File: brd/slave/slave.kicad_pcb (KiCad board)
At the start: 2 copper layers, 43.2 x 25.4 mm, 23 parts, among them P1 CONN_3X2, P2 CONN_8, P3 CONN_2, P4 CONN_6, P5 CONN_1, Q1 BC847, U1 LM78L05ACZ, U2 ATMEGA328P-A, X1 16MHz

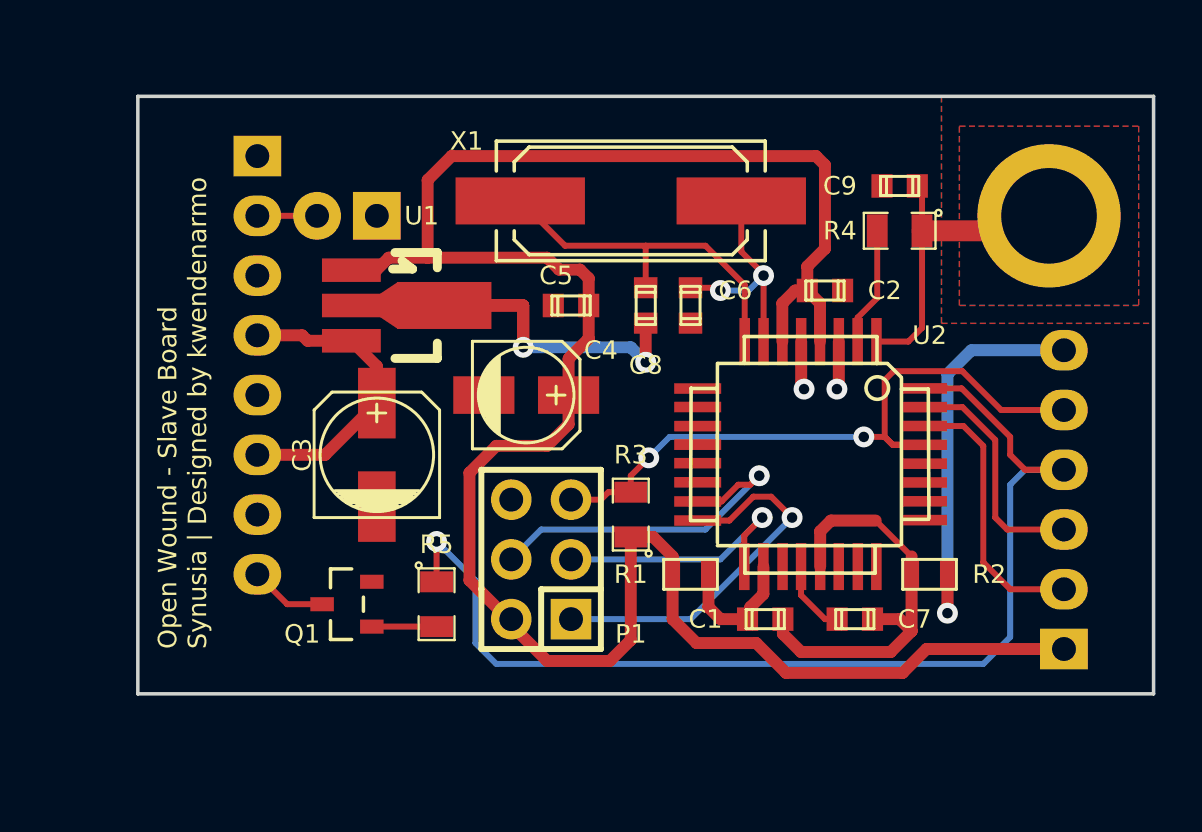
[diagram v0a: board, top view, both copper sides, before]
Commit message: slave version rc3
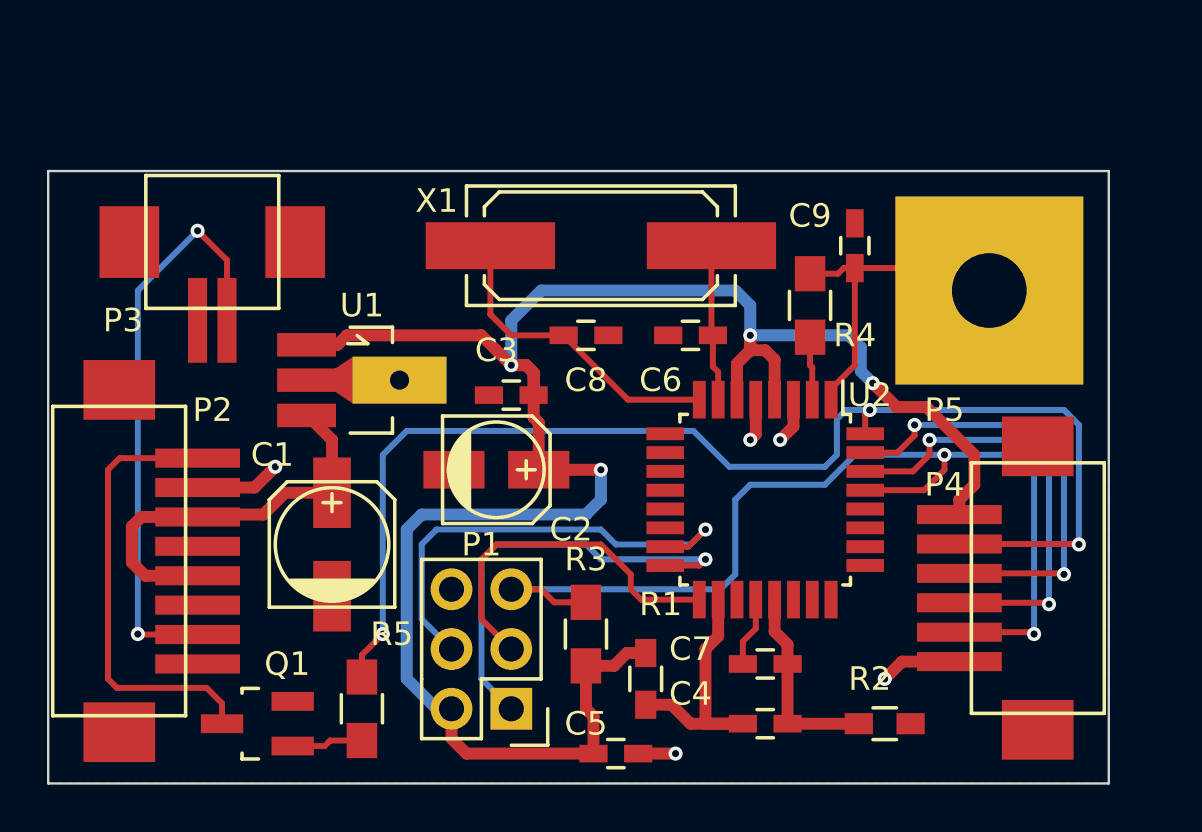
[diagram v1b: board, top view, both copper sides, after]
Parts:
- added REF**: Symbol_OSHW-Logo_SilkScreen, Symbols:Symbol_OSHW-Logo_SilkScreen, B.Cu at (157.5, 103.5)
- C1: value 100nF -> 10uF; footprint Capacitors_SMD:c_0603 -> Capacitors_SMD:c_elec_5x5.3
- C2: value 100nF -> 1uF; footprint Capacitors_SMD:c_0603 -> Capacitors_SMD:c_elec_4x5.3
- C3: value 10uF -> 10nF; footprint Capacitors_SMD:c_elec_5x5.3 -> Capacitors_SMD:C_0603_HandSoldering
- C4: value 1uF -> 100nF; footprint Capacitors_SMD:c_elec_4x5.3 -> Capacitors_SMD:C_0603_HandSoldering
- C5: value 10nF -> 100nF; footprint Capacitors_SMD:c_0603 -> Capacitors_SMD:C_0603_HandSoldering
- C6, C7, C8, C9: footprint Capacitors_SMD:c_0603 -> Capacitors_SMD:C_0603_HandSoldering
- P1: value CONN_3X2 -> AVRISP
- P2: value CONN_8 -> IO; footprint Pin_Headers:Pin_Header_Straight_1x08 -> asrdi-conn:IL-Z-8PL-SMTYE; moved to F.Cu
- P3: value CONN_2 -> PIEZO; footprint Pin_Headers:Pin_Header_Straight_1x02 -> asrdi-conn:IL-Z-2PL-SMTYE; moved to F.Cu
- P4: value CONN_6 -> DEBUG; footprint Pin_Headers:Pin_Header_Straight_1x06 -> asrdi-conn:IL-Z-6PL-SMTYE; moved to F.Cu
- P5: value CONN_1 -> SENSE
- Q1: footprint Transistors_SMD:sot23 -> Housings_SOT-23_SOT-143_TSOT-6:SOT-23_Handsoldering
- R1, R2: footprint SMD_Packages:SM0603 -> Resistors_SMD:R_0603_HandSoldering
- R3, R4, R5: footprint SMD_Packages:SM0805 -> Resistors_SMD:R_0805_HandSoldering
- U2: footprint SMD_Packages:TQFP32 -> Housings_QFP:TQFP-32_7x7mm_Pitch0.8mm
- moved C5 19.1 mm to (151.1, 114.3)
- moved C1 18.7 mm to (139.1, 105.4), turned to 90 degrees
- moved C4 17.3 mm to (157.5, 113.0)
- moved C2 15.9 mm to (146.1, 102.2), turned to 0 degrees
- moved P2 13.0 mm to (133.3, 110.5), turned to 180 degrees
- moved P3 7.75 mm to (133.3, 95.9), turned to 90 degrees
- moved R2 6.63 mm to (162.6, 113.0)
- moved P1 6.48 mm to (146.7, 112.4), turned to 180 degrees
- moved Q1 6.35 mm to (135.9, 113.0)
- moved C3 6.25 mm to (146.7, 99.1), turned to 180 degrees
- moved R5 5.46 mm to (140.3, 112.4)
- moved R3 5.43 mm to (149.9, 109.2)
- moved R4 4.96 mm to (159.4, 95.2), turned to 270 degrees
- moved R1 4.84 mm to (152.4, 111.1), turned to 270 degrees
- moved P4 4.49 mm to (165.7, 104.1), turned to 0 degrees
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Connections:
- C1 pad 1: +5VA -> VCC
- C1 pad 2: AGND -> GND
- C3 pad 1: VCC -> +5V
- C4 pad 1: +5V -> +5VA
- C4 pad 2: GND -> GNDA
- C7 pad 2: AGND -> GNDA
- R2 pad 2: AGND -> GNDA
- R5 pad 1: Net-(P4-Pad4) -> Net-(P4-Pad2)
- U2 pad 21: AGND -> GNDA
- U2 pad 30: Net-(P4-Pad2) -> Net-(P4-Pad4)
- U2 pad 32: Net-(P4-Pad4) -> Net-(P4-Pad2)
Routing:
- net Net-(P4-Pad2): track 11.7 -> 53.9 mm, vias 0 -> 3
- net Net-(P4-Pad4): track 47.2 -> 19.3 mm, vias 1 -> 2
- net GND: track 38.9 -> 12.5 mm
- net Net-(P2-Pad2): track 2.54 -> 25.1 mm, vias 0 -> 2
- net AGND: track 18.0 -> 0.00 mm
- net Net-(P1-Pad5): track 29.3 -> 45.4 mm
- net Net-(P2-Pad8): track 3.28 -> 19.1 mm
- net Net-(P4-Pad3): track 10.1 -> 19.6 mm, vias 0 -> 2
- net GNDA: track 0.00 -> 8.53 mm
- net +5V: track 94.6 -> 88.1 mm, vias 0 -> 4
- net Net-(P1-Pad4): track 15.1 -> 21.0 mm
- net +5VA: track 5.78 -> 11.6 mm
- net VCC: track 13.2 -> 17.4 mm
- net Net-(P1-Pad3): track 11.3 -> 15.2 mm, vias 1 -> 0
- net Net-(C6-Pad1): track 9.79 -> 6.66 mm, vias 2 -> 0
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- removed copper zone on B.Cu, net Net-(C9-Pad1)
- removed copper zone on F.Cu, net Net-(C9-Pad1)
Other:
- board size 43.2 x 25.4 mm -> 45.1 x 26 mm
- net class Default: clearance 0.254 -> 0.2032; via_dia 0.889 -> 0.59944; via_drill 0.635 -> 0.39878
- net class Power: clearance 0.254 -> 0.2032; via_dia 0.889 -> 0.59944; via_drill 0.635 -> 0.39878
- net class Sense removed
- rule trace_clearance: 0.254 -> 0.2032
- rule trace_min: 0.254 -> 0.2032
- rule via_min_drill: 0.508 -> 0.29972
- rule via_min_size: 0.889 -> 0.39878
- board text added: "Open Wound - Slave board rc3 Synusia | Designed by kwendenarmo https://github.com/synusia/open-wound UNDER MIT LICENSE"
- board text removed: "Open Wound - Slave Board Synusia | Designed by kwendenarmo"
